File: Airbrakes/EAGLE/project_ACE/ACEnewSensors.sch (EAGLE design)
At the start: 24 parts, among them J3 PTH, U2 MPM3630GQV-P

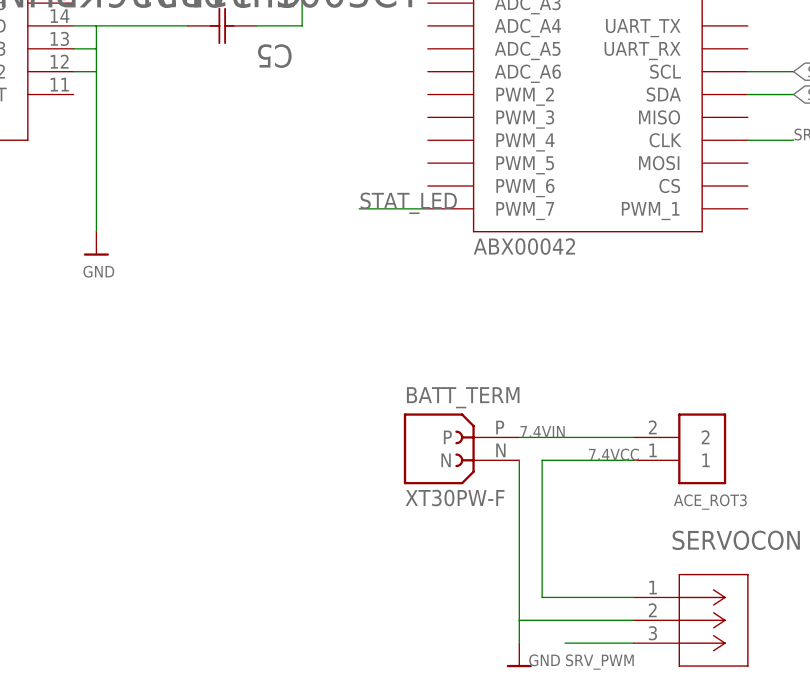
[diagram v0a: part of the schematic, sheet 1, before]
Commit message: Finalize PACE board
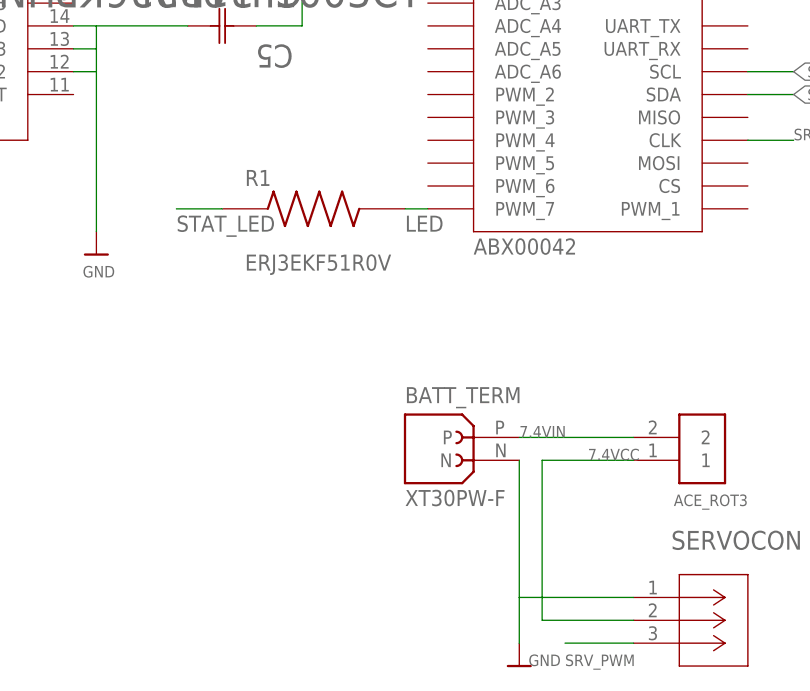
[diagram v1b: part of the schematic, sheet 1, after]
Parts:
- added R1: ERJ3EKF51R0V, ERJ3EKF51R0V-51Ohm-Resistor:ERJ3EKF51R0V
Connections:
- new net LED: R1.2, U$10.PWM_7
- net 7.4VCC: now also SERVOCON.2; no longer SERVOCON.1
- net GND: now also SERVOCON.1; no longer SERVOCON.2
- net STAT_LED: now also R1.1; no longer U$10.PWM_7
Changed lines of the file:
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@@
 <part name="SUPPLY4" library="supply2" library_urn="urn:adsk.eagle:library:372" deviceset="AGND" device=""/>
 <part name="ACE_ROT3" library="282837-2" deviceset="282837-2" device=""/>
+<part name="R1" library="ERJ3EKF51R0V-51Ohm-Resistor" deviceset="ERJ3EKF51R0V" device=""/>
 </parts>
 <sheets>
@@
 <attribute name="NAME" x="20.319440625" y="5.07618125" size="1.271909375" layer="95" rot="MR0"/>
 </instance>
+<instance part="R1" gate="G$1" x="-27.94" y="38.1" smashed="yes">
+<attribute name="NAME" x="-35.564" y="40.641" size="1.778" layer="95"/>
+<attribute name="VALUE" x="-35.564" y="33.013" size="1.778" layer="96" align="top-left"/>
+</instance>
 </instances>
 <busses>
@@
 </segment>
 <segment>
-<pinref part="SERVOCON" gate="A" pin="2"/>
-<wire x1="7.62" y1="-7.62" x2="-5.08" y2="-7.62" width="0.1524" layer="91"/>
 <pinref part="U$6" gate="G$1" pin="GND"/>
-<wire x1="-5.08" y1="-10.16" x2="-5.08" y2="-7.62" width="0.1524" layer="91"/>
-<wire x1="-5.08" y1="10.16" x2="-5.08" y2="-7.62" width="0.1524" layer="91"/>
+<wire x1="-5.08" y1="10.16" x2="-5.08" y2="-5.08" width="0.1524" layer="91"/>
 <pinref part="BATT_TERM" gate="G$1" pin="N"/>
+<pinref part="SERVOCON" gate="A" pin="1"/>
+<wire x1="-5.08" y1="-5.08" x2="-5.08" y2="-10.16" width="0.1524" layer="91"/>
+<wire x1="7.62" y1="-5.08" x2="-5.08" y2="-5.08" width="0.1524" layer="91"/>
 </segment>
 <segment>
@@
 <net name="7.4VCC" class="0">
 <segment>
-<pinref part="SERVOCON" gate="A" pin="1"/>
 <label x="2.54" y="10.16" size="1.27" layer="95"/>
-<wire x1="7.62" y1="-5.08" x2="-2.54" y2="-5.08" width="0.1524" layer="91"/>
-<wire x1="-2.54" y1="-5.08" x2="-2.54" y2="10.16" width="0.1524" layer="91"/>
+<wire x1="-2.54" y1="-7.62" x2="-2.54" y2="10.16" width="0.1524" layer="91"/>
 <wire x1="7.62" y1="10.16" x2="-2.54" y2="10.16" width="0.1524" layer="91"/>
 <pinref part="ACE_ROT3" gate="G$1" pin="1"/>
+<pinref part="SERVOCON" gate="A" pin="2"/>
+<wire x1="-2.54" y1="-7.62" x2="7.62" y2="-7.62" width="0.1524" layer="91"/>
 </segment>
 <segment>
@@
 </segment>
 </net>
+<net name="LED" class="0">
+<segment>
+<pinref part="U$10" gate="G$1" pin="PWM_7"/>
+<pinref part="R1" gate="G$1" pin="2"/>
+<wire x1="-17.78" y1="38.1" x2="-15.24" y2="38.1" width="0.1524" layer="91"/>
+<label x="-17.78" y="35.56" size="1.778" layer="95"/>
+</segment>
+</net>
 <net name="STAT_LED" class="0">
 <segment>
-<pinref part="U$10" gate="G$1" pin="PWM_7"/>
-<wire x1="-15.24" y1="38.1" x2="-22.86" y2="38.1" width="0.1524" layer="91"/>
-<label x="-22.86" y="38.1" size="1.778" layer="95"/>
-</segment>
-</net>
+<pinref part="R1" gate="G$1" pin="1"/>
+<wire x1="-38.1" y1="38.1" x2="-43.18" y2="38.1" width="0.1524" layer="91"/>
+<label x="-43.18" y="35.56" size="1.778" layer="95"/>
+</segment>
+</net>
